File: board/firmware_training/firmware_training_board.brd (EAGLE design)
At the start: 54 x 45 mm, 16 parts, among them J1 GY-521-MPU-6050, SW1 PTS645, SW2 PTS645

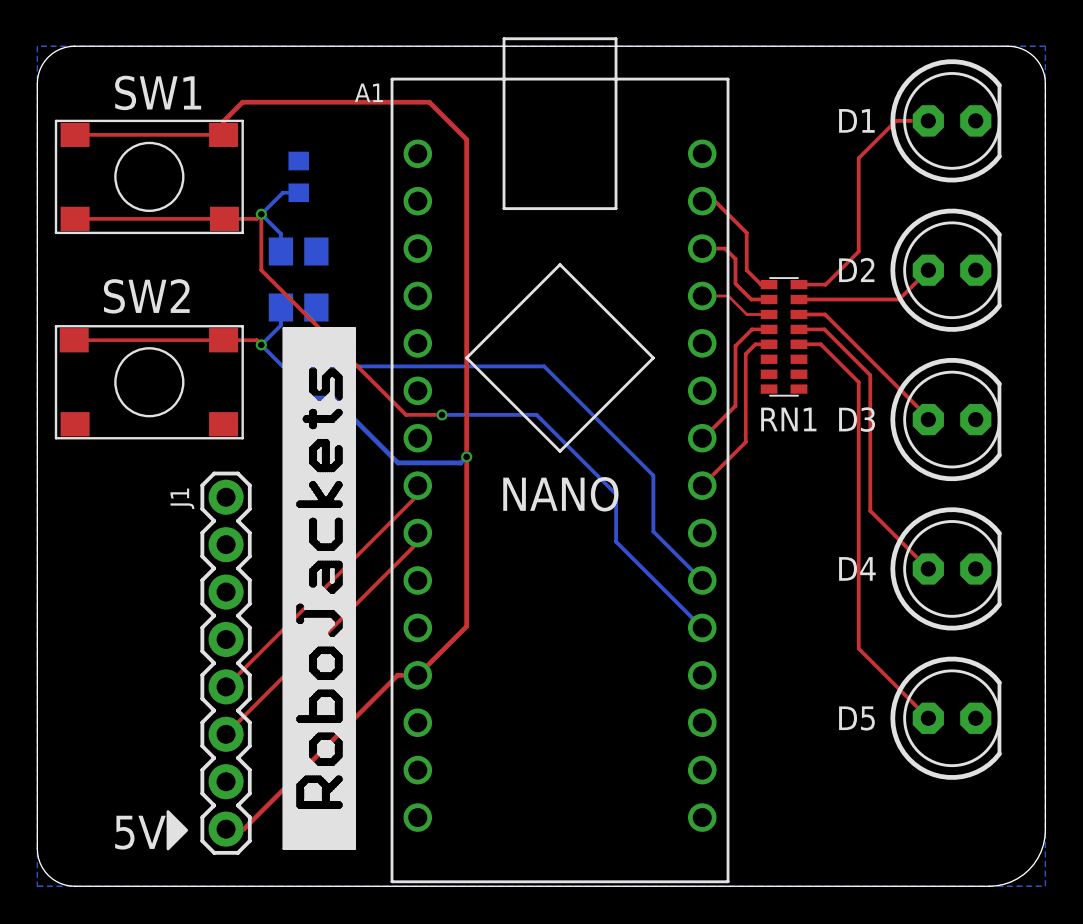
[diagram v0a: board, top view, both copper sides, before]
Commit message: Moved parts to top
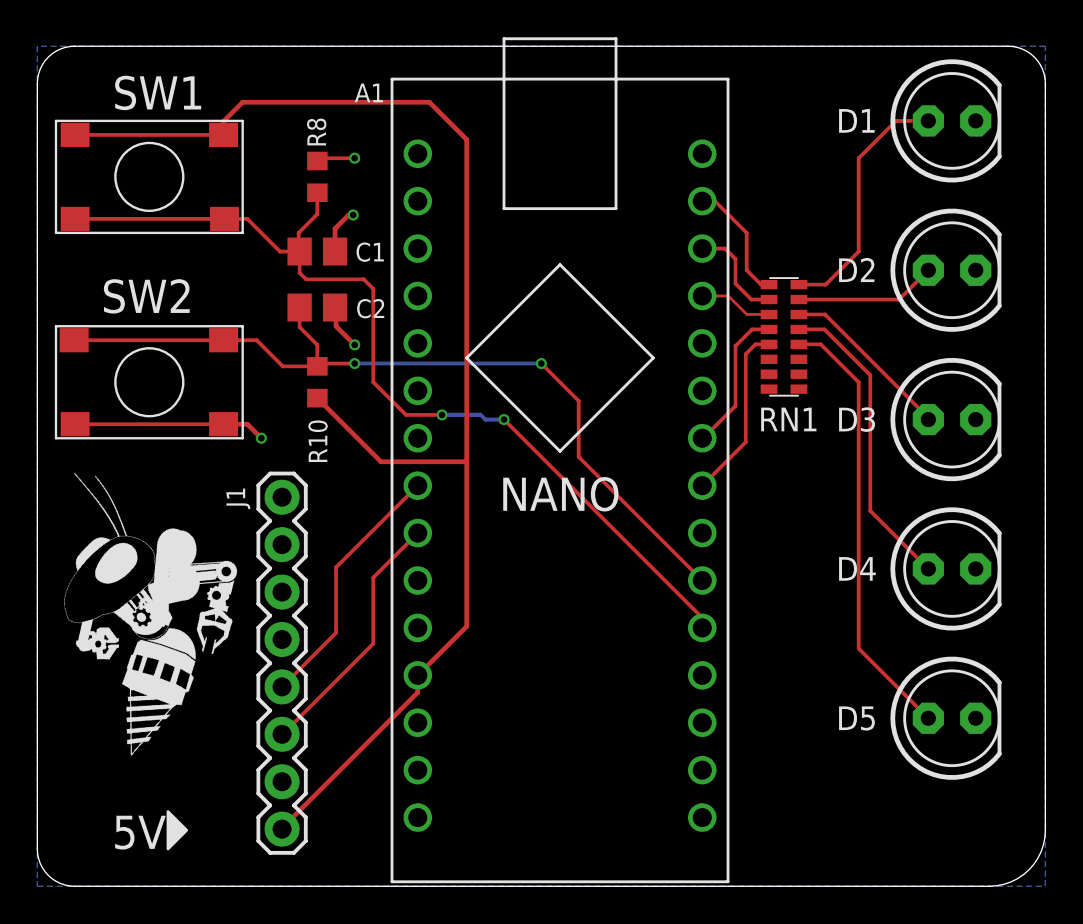
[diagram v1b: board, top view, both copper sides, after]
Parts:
- moved U$3 22.8 mm to (39.0, 8.00), flipped to the bottom
- moved U$4 22.2 mm to (5.00, 7.00), flipped to the top
- moved J1 3.00 mm to (13.1, 3.06)
- moved C1 1.00 mm to (15.0, 34.0), flipped to the top, turned to 0 degrees
- moved C2 1.00 mm to (15.0, 31.0), flipped to the top, turned to 0 degrees
- moved R10 1.00 mm to (15.0, 27.0), flipped to the top
- moved R8 1.00 mm to (15.0, 38.0), flipped to the top
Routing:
- net GND: track 0.00 -> 17.3 mm, vias 0 -> 4
- net +5V: track 77.0 -> 73.4 mm, vias 1 -> 0
- net SDA: track 15.0 -> 13.8 mm
- net SCL: track 15.0 -> 13.8 mm
- net !SW2_INPUT: track 43.2 -> 44.3 mm, vias 1 -> 2
- net SW1_INT: track 51.0 -> 50.2 mm
